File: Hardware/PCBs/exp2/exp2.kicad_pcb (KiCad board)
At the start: 2 copper layers, 44.5 x 47 mm, 8 parts, among them J1 Conn_01x11_Female, J2 Conn_01x06_Female, U1 74HC86, U2 7483

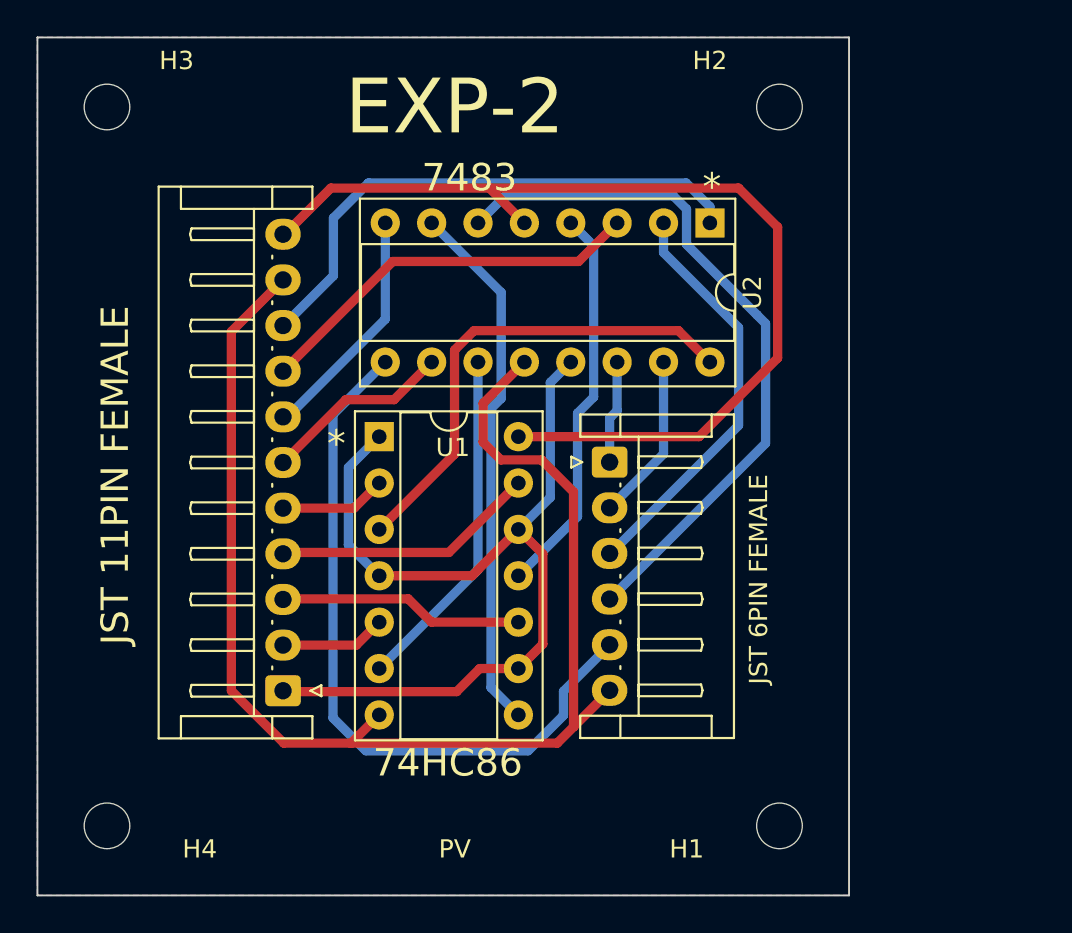
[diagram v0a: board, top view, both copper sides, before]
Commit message: Exp - 2 and 3 PCB Updated
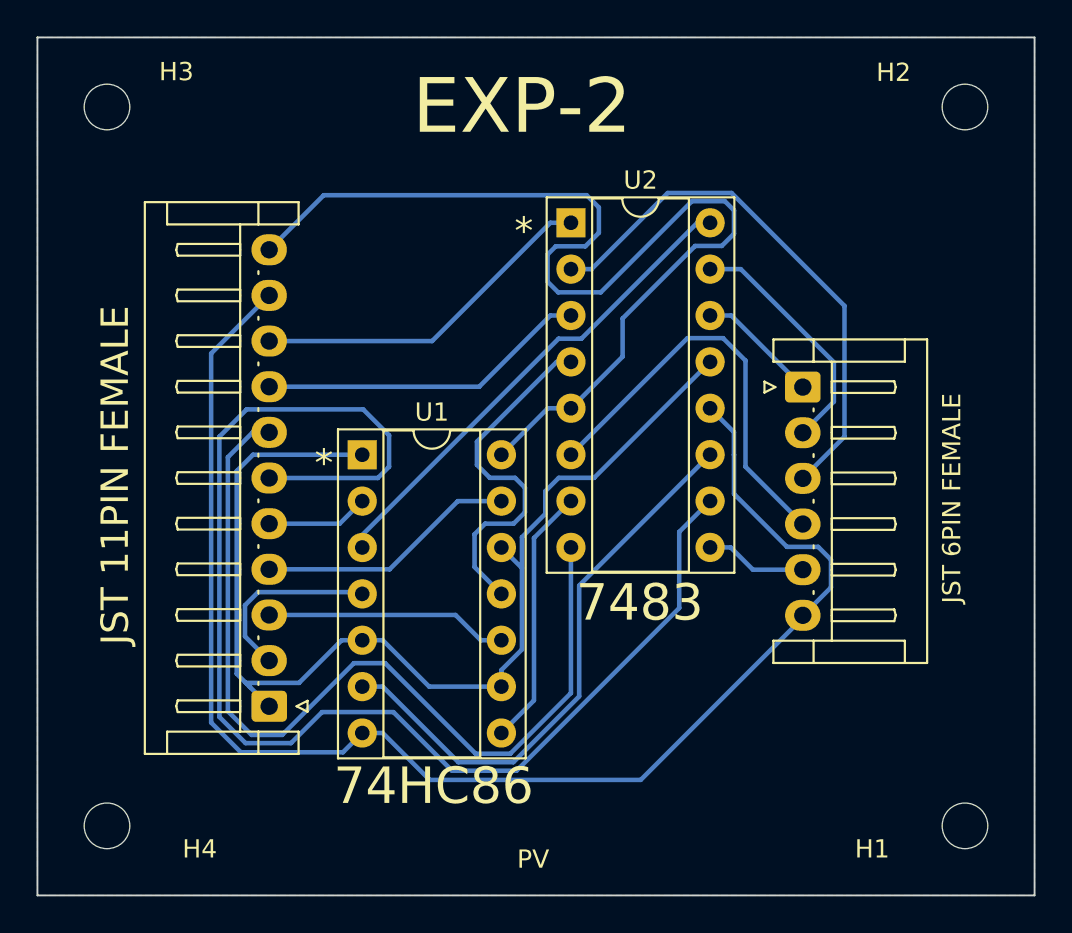
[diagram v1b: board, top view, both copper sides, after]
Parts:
- moved J2 11.4 mm to (139.7, 95.3)
- moved H1 10.2 mm to (148.6, 119.4)
- moved H2 10.2 mm to (148.6, 80.0)
- moved U2 7.61 mm to (127.0, 86.3), turned to 0 degrees
- moved U1 1.36 mm to (115.6, 99.1)
- moved J1 1.14 mm to (110.5, 112.8)
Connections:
- U1 pad 4: Cin -> B0
- U1 pad 5: B0 -> Cin
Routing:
- net A0: track 10.4 -> 72.5 mm
- net A1: track 13.1 -> 49.1 mm
- net S0: track 39.7 -> 5.58 mm
- net S1: track 39.0 -> 23.0 mm
- net Net-(U1-Pad8): track 29.4 -> 14.3 mm
- net Net-(U1-Pad6): track 19.0 -> 31.3 mm
- net Cin: track 50.2 -> 62.2 mm
- net A3: track 29.9 -> 19.2 mm
- net S2: track 22.8 -> 29.7 mm
- net GND: track 73.2 -> 78.8 mm
- net B0: track 5.79 -> 10.3 mm
- net S3: track 9.20 -> 13.5 mm
- net VCC: track 54.9 -> 58.7 mm
- net A2: track 21.7 -> 18.1 mm
- net Net-(U1-Pad11): track 21.6 -> 19.9 mm
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- removed copper zone on F.Cu, net (none)
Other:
- board size 44.5 x 47 mm -> 54.6 x 47 mm
